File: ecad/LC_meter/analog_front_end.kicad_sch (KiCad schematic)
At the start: 56 parts, among them J1 DUT, Q1 2N7000, Q2 2N7000, SW1 SW_SP3T, U1 LMC6484, U2 LMC6482, U3 MCP3204, U4 LM385BZ-2.5, U6 LTC1044

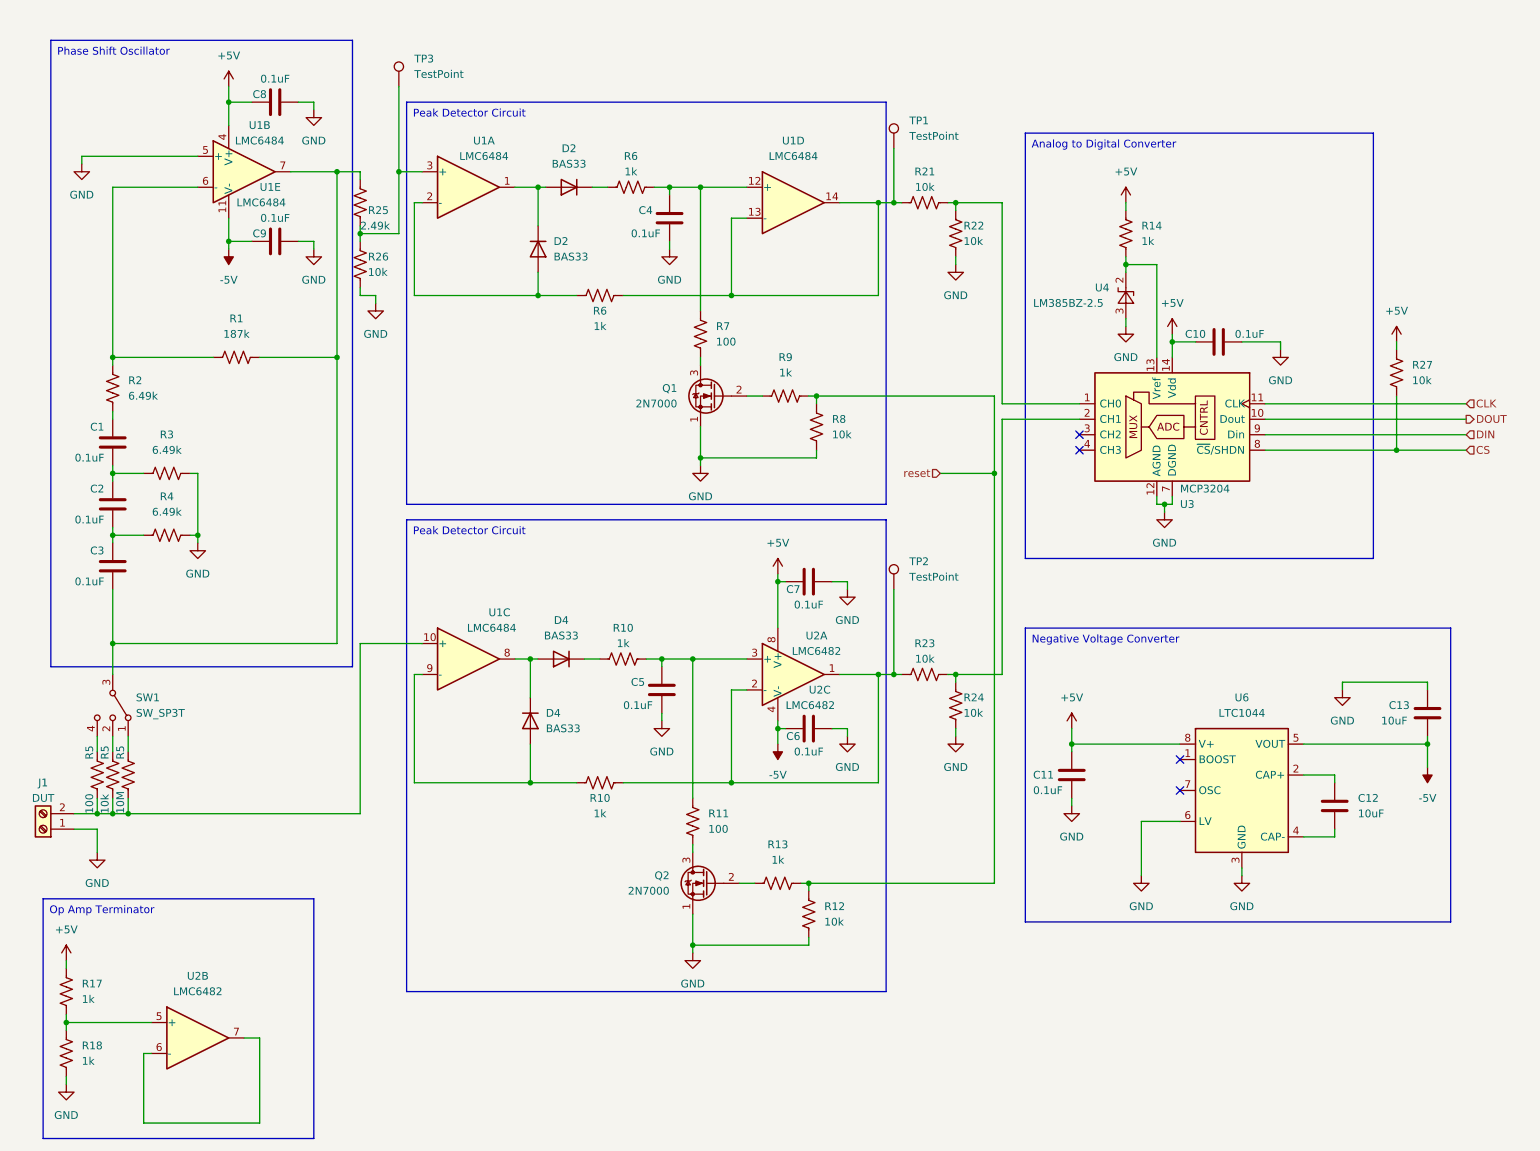
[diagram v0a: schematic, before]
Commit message: new computer
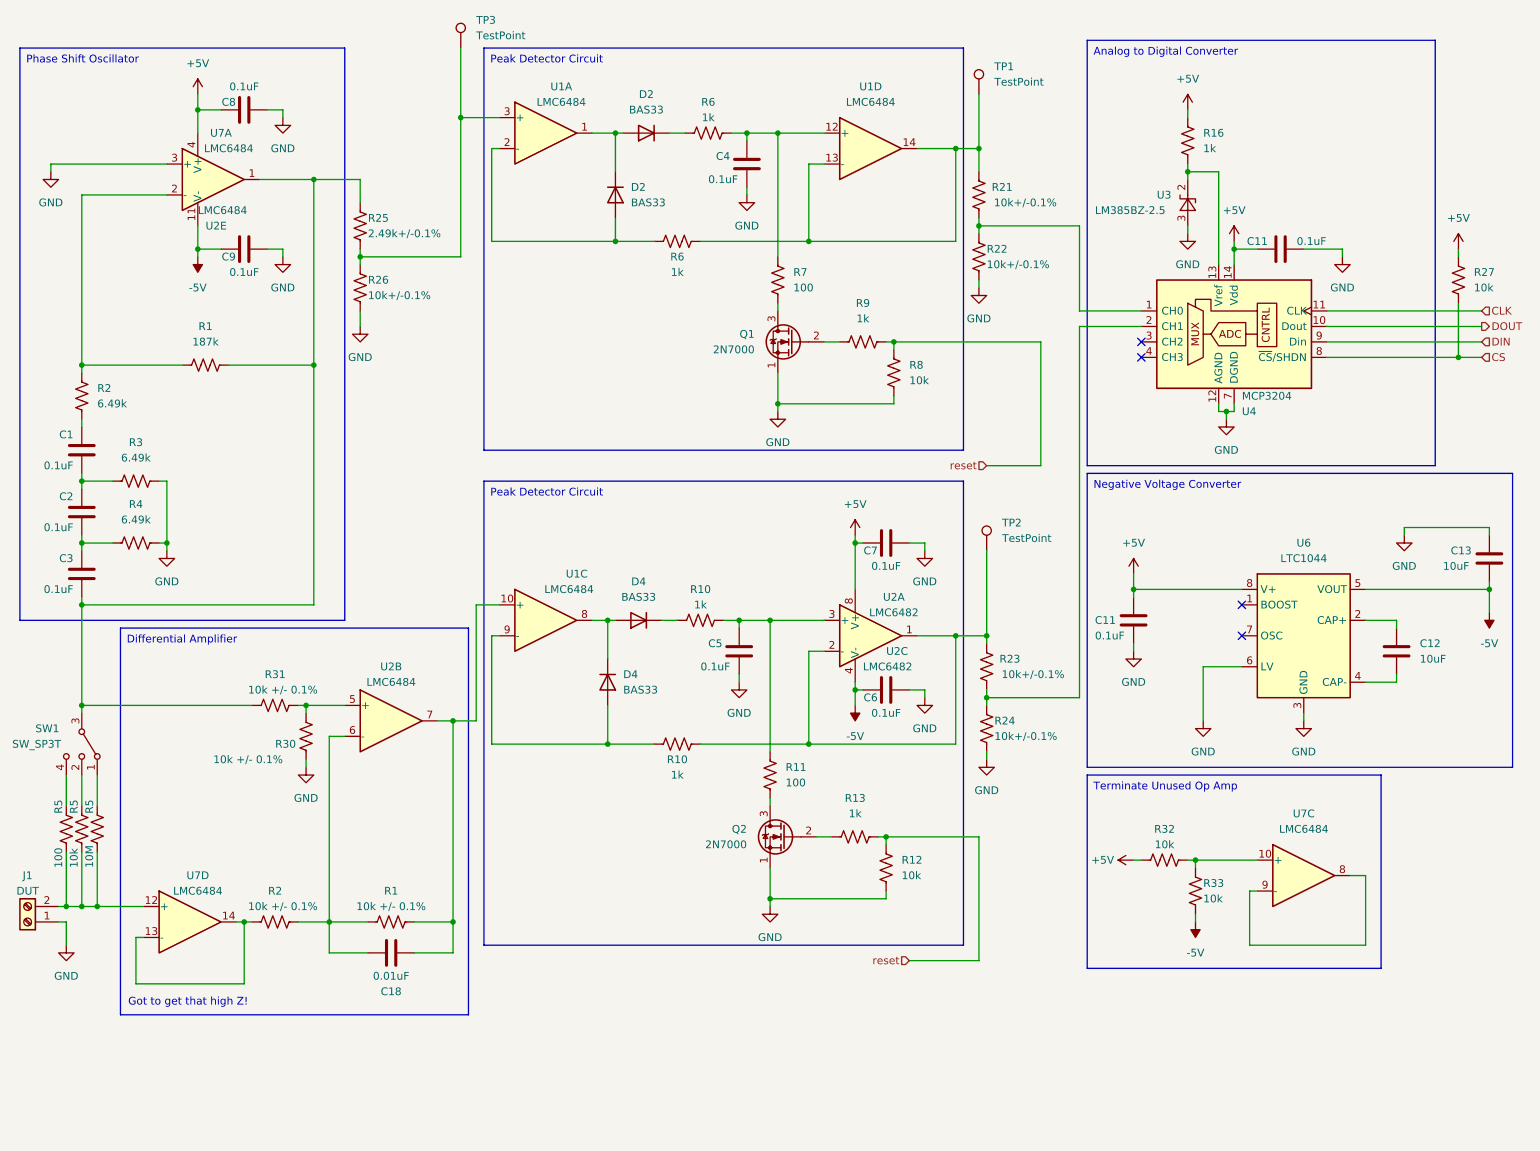
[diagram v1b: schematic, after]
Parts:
- removed C10: 0.1uF, symbol Device:C
- removed R14, R17, R18: 1k, symbol Device:R_US
- removed unit 5 of U1
- removed unit 2 of U1
- removed unit 2 of U2
- removed U3: MCP3204, symbol Analog_ADC:MCP3204
- removed U4: LM385BZ-2.5, Package_TO_SOT_THT:TO-92_Inline, symbol Reference_Voltage:LM385BZ-2.5
- added C11: 0.1uF, symbol Device:C
- added C18: 0.01uF, symbol Device:C
- added R1, R2, R30, R31: 10k +/- 0.1%, symbol Device:R_US
- added R16: 1k, symbol Device:R_US
- added R32, R33: 10k, symbol Device:R_US
- added unit 2 of U2
- added unit 5 of U2
- added U3: LM385BZ-2.5, Package_TO_SOT_THT:TO-92_Inline, symbol Reference_Voltage:LM385BZ-2.5
- added U4: MCP3204, symbol Analog_ADC:MCP3204
- added U7: LMC6484, symbol Amplifier_Operational:LMC6484
- R21, R22, R23, R24, R26: value 10k -> 10k+/-0.1%
- R25: value 2.49k -> 2.49k+/-0.1%
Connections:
- net +5V: now also C11.1, R16.1, R32.1, U2.4 (V+), U4.14 (Vdd)
- net -5V: now also R33.1, U2.11 (V-)
- net CLK: now also U4.11 (CLK)
- net CS: now also U4.8 (~{CS}/SHDN)
- net DIN: now also U4.9 (Din)
- net DOUT: now also U4.10 (Dout)
- net GND: now also C11.2, R30.2, U3.3 (A), U4.12 (AGND), U4.7 (DGND), U7.3 (+)
- net at R21.2, R22.2: now also U4.1 (CH0)
- net at C3.1, R1.2, R25.1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: now also R31.1, U7.1
- net at R1.1, R2.2: now also U7.2 (-)
- net at J1.2 (Pin_2), R5.2, R5.2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: now also U7.12 (+); no longer U1.10 (+)
- net at R23.2, R24.2: now also U4.2 (CH1)
- new net: C18.2, R1.1, R2.2, U2.6 (-)
- new net: C18.1, R1.2, U1.10 (+), U2.7
- new net: R30.1, R31.2, U2.5 (+)
- new net: R2.1, U7.13 (-), U7.14
- new net: R32.2, R33.2, U7.10 (+)
- new net: R16.2, U3.2 (K), U4.13 (Vref)
- new net: U7.8, U7.9 (-)
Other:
- note added: "Got to get that high Z!"
- moved on the sheet: C1, C11, C12, C13, C2, C3, C4, C5, C6, C7, C8, C9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
